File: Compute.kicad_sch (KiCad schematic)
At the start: 11 parts, among them J1 Conn_ARM_JTAG_SWD_10, U3 STM32C542CCT6, Y2 32.768kHz

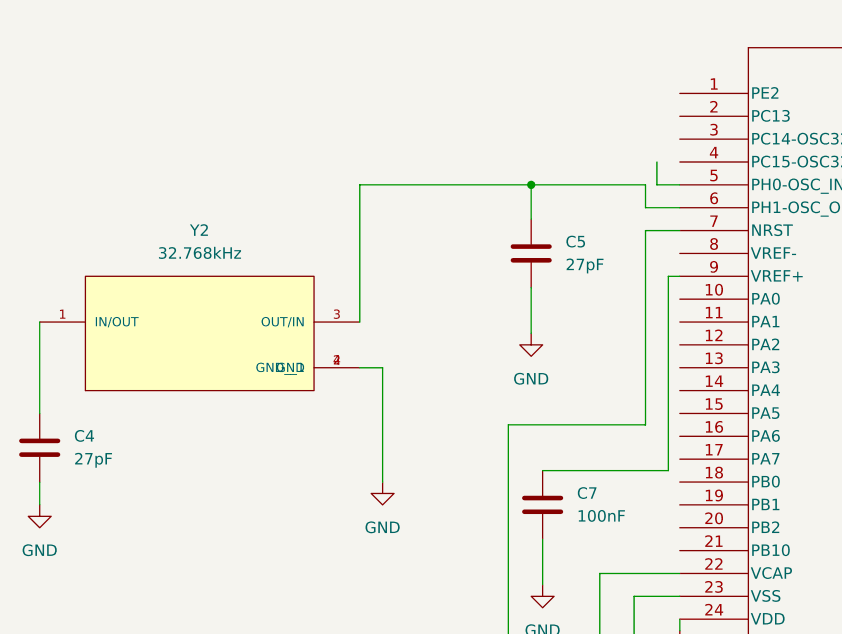
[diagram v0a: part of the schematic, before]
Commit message: fixed stuff
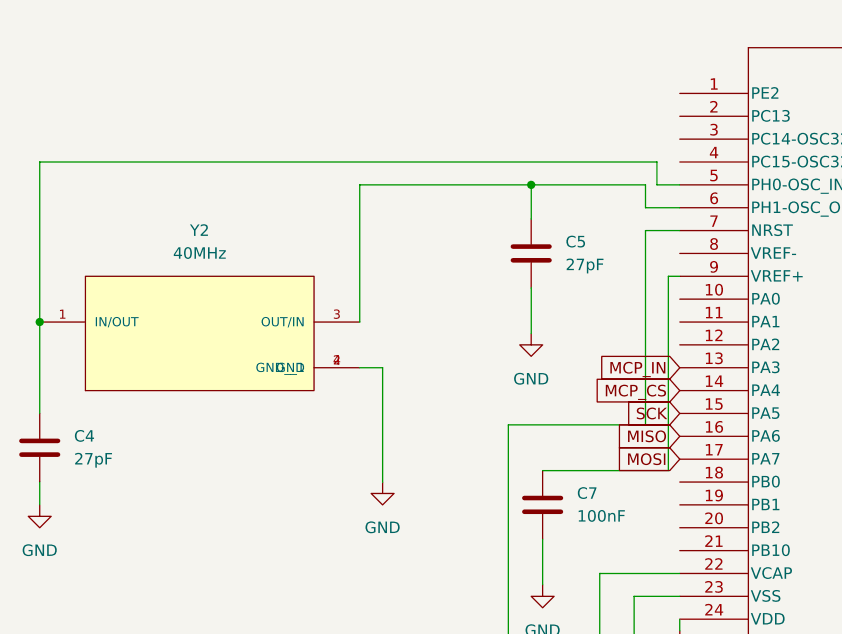
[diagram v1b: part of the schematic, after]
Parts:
- Y2: value 32.768kHz -> 40MHz
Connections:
- net MCP_IN: now reaches U3.13 (PA3)
- net MCP_CS: now reaches U3.14 (PA4)
- net SCK: now reaches U3.15 (PA5)
- net MISO: now reaches U3.16 (PA6)
- net MOSI: now reaches U3.17 (PA7)
- net at U3.5 (PH0-OSC_IN): now also C4.1, Y2.1 (IN/OUT)
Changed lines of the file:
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@@
+	)
+	(junction
+		(at 41.91 68.58)
+		(diameter 0)
+		(color 0 0 0 0)
 	)
 	(junction
@@
 	(wire
 		(pts
+			(xy 110.49 53.34) (xy 113.03 53.34)
+		)
+		(stroke
+			(width 0)
+			(type default)
+		)
+	)
+	(wire
+		(pts
 			(xy 97.79 85.09) (xy 111.76 85.09)
 		)
@@
 	(wire
 		(pts
+			(xy 110.49 50.8) (xy 110.49 53.34)
+		)
+		(stroke
+			(width 0)
+			(type default)
+		)
+	)
+	(wire
+		(pts
 			(xy 184.15 45.72) (xy 194.31 45.72)
 		)
@@
 	(wire
 		(pts
-			(xy 110.49 53.34) (xy 113.03 53.34)
-		)
-		(stroke
-			(width 0)
-			(type default)
-		)
-	)
-	(wire
-		(pts
-			(xy 110.49 50.8) (xy 110.49 53.34)
-		)
-		(stroke
-			(width 0)
-			(type default)
-		)
-	)
-	(wire
-		(pts
 			(xy 231.14 106.68) (xy 231.14 77.47)
 		)
@@
 	(wire
 		(pts
+			(xy 41.91 50.8) (xy 110.49 50.8)
+		)
+		(stroke
+			(width 0)
+			(type default)
+		)
+	)
+	(wire
+		(pts
 			(xy 184.15 76.2) (xy 186.69 76.2)
 		)
@@
 			(width 0)
 			(type default)
+		)
+	)
+	(wire
+		(pts
+			(xy 41.91 68.58) (xy 41.91 50.8)
+		)
+		(stroke
+			(width 0)
+			(type default)
+		)
+	)
+	(global_label "MCP_CS"
+		(shape input)
+		(at 113.03 76.2 180)
+		(fields_autoplaced yes)
+		(effects
+			(font
+				(size 1.27 1.27)
+			)
+			(justify right)
+		)
+		(property "Intersheetrefs" "${INTERSHEET_REFS}"
+			(at 102.6063 76.2 0)
+			(hide yes)
+			(show_name no)
+			(do_not_autoplace no)
+			(effects
+				(font
+					(size 1.27 1.27)
+				)
+				(justify right)
+			)
 		)
 	)
@@
 		)
 	)
+	(global_label "MCP_IN"
+		(shape input)
+		(at 113.03 73.66 180)
+		(fields_autoplaced yes)
+		(effects
+			(font
+				(size 1.27 1.27)
+			)
+			(justify right)
+		)
+		(property "Intersheetrefs" "${INTERSHEET_REFS}"
+			(at 103.1505 73.66 0)
+			(hide yes)
+			(show_name no)
+			(do_not_autoplace no)
+			(effects
+				(font
+					(size 1.27 1.27)
+				)
+				(justify right)
+			)
+		)
+	)
+	(global_label "MISO"
+		(shape input)
+		(at 113.03 81.28 180)
+		(fields_autoplaced yes)
+		(effects
+			(font
+				(size 1.27 1.27)
+			)
+			(justify right)
+		)
+		(property "Intersheetrefs" "${INTERSHEET_REFS}"
+			(at 105.4486 81.28 0)
+			(hide yes)
+			(show_name no)
+			(do_not_autoplace no)
+			(effects
+				(font
+					(size 1.27 1.27)
+				)
+				(justify right)
+			)
+		)
+	)
 	(global_label "CAN_RX"
 		(shape input)
@@
 				)
 				(justify left)
+			)
+		)
+	)
+	(global_label "MOSI"
+		(shape input)
+		(at 113.03 83.82 180)
+		(fields_autoplaced yes)
+		(effects
+			(font
+				(size 1.27 1.27)
+			)
+			(justify right)
+		)
+		(property "Intersheetrefs" "${INTERSHEET_REFS}"
+			(at 105.4486 83.82 0)
+			(hide yes)
+			(show_name no)
+			(do_not_autoplace no)
+			(effects
+				(font
+					(size 1.27 1.27)
+				)
+				(justify right)
+			)
+		)
+	)
+	(global_label "SCK"
+		(shape input)
+		(at 113.03 78.74 180)
+		(fields_autoplaced yes)
+		(effects
+			(font
+				(size 1.27 1.27)
+			)
+			(justify right)
+		)
+		(property "Intersheetrefs" "${INTERSHEET_REFS}"
+			(at 106.2953 78.74 0)
+			(hide yes)
+			(show_name no)
+			(do_not_autoplace no)
+			(effects
+				(font
+					(size 1.27 1.27)
+				)
+				(justify right)
 			)
 		)
@@
 			)
 		)
-		(property "Value" "32.768kHz"
+		(property "Value" "40MHz"
 			(at 59.69 60.96 0)
 			(show_name no)

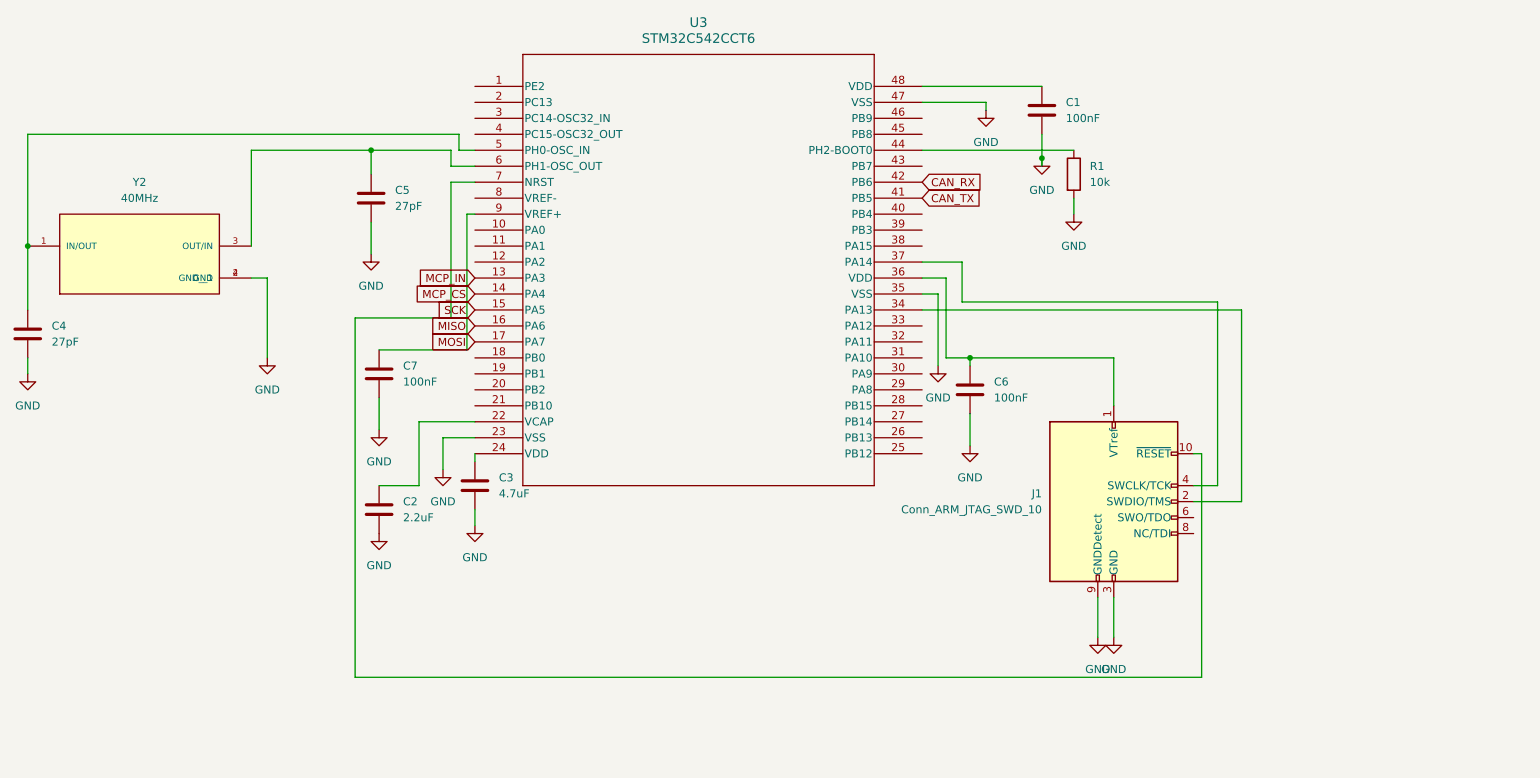
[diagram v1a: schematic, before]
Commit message: more fixes
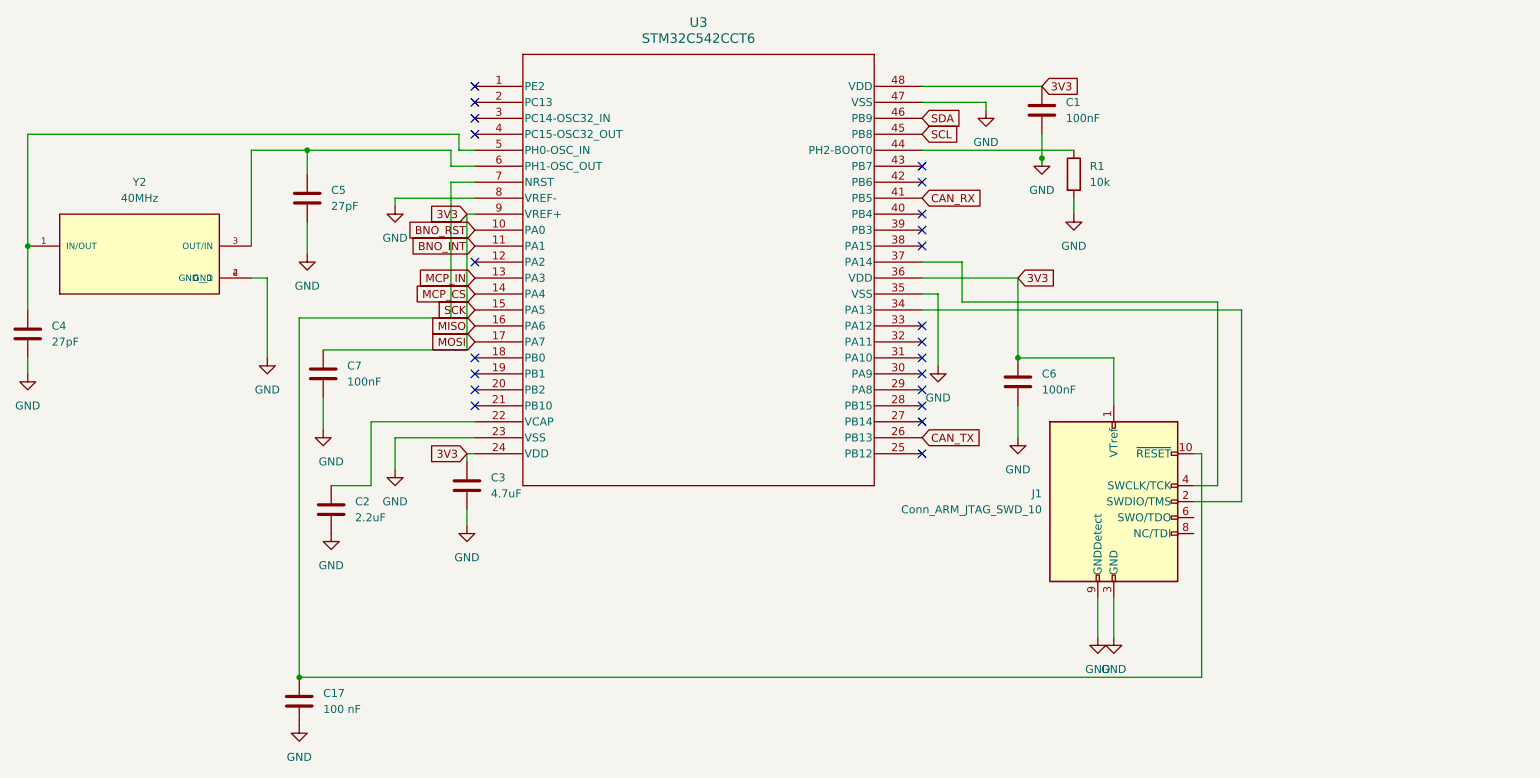
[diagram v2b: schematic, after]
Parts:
- added C17: 100 nF, symbol Device:C
- C1, C2, C3, C4, C5: footprint rov_power:SOT-23-5_MC_MCH -> Capacitor_SMD:C_0201_0603Metric
- C6, C7: footprint (none) -> Capacitor_SMD:C_0201_0603Metric
- J1: footprint (none) -> Connector_PinHeader_1.27mm:PinHeader_2x05_P1.27mm_Vertical
- R1: footprint rov_logic:LQFP48-7X7 -> Resistor_SMD:R_0201_0603Metric
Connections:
- net CAN_RX: now also U3.41 (PB5); no longer U3.42 (PB6)
- net CAN_TX: now also U3.26 (PB13); no longer U3.41 (PB5)
- net GND: now also U3.8 (VREF-), C17.2
- net 3V3: now reaches C7.1, U3.9 (VREF+)
- net 3V3: now also C1.1, C3.1, C6.1, J1.1 (VTref), U3.24 (VDD), U3.36 (VDD), U3.48 (VDD)
- net BNO_RST: now reaches U3.10 (PA0)
- net BNO_INT: now reaches U3.11 (PA1)
- net SCL: now reaches U3.45 (PB8)
- net SDA: now reaches U3.46 (PB9)
- net at J1.10 (~{RESET}), U3.7 (NRST): now also C17.1
- no-connect marks 0 -> 22
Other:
- moved on the sheet: C2, C3, C5, C6, C7

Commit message: i did stuff
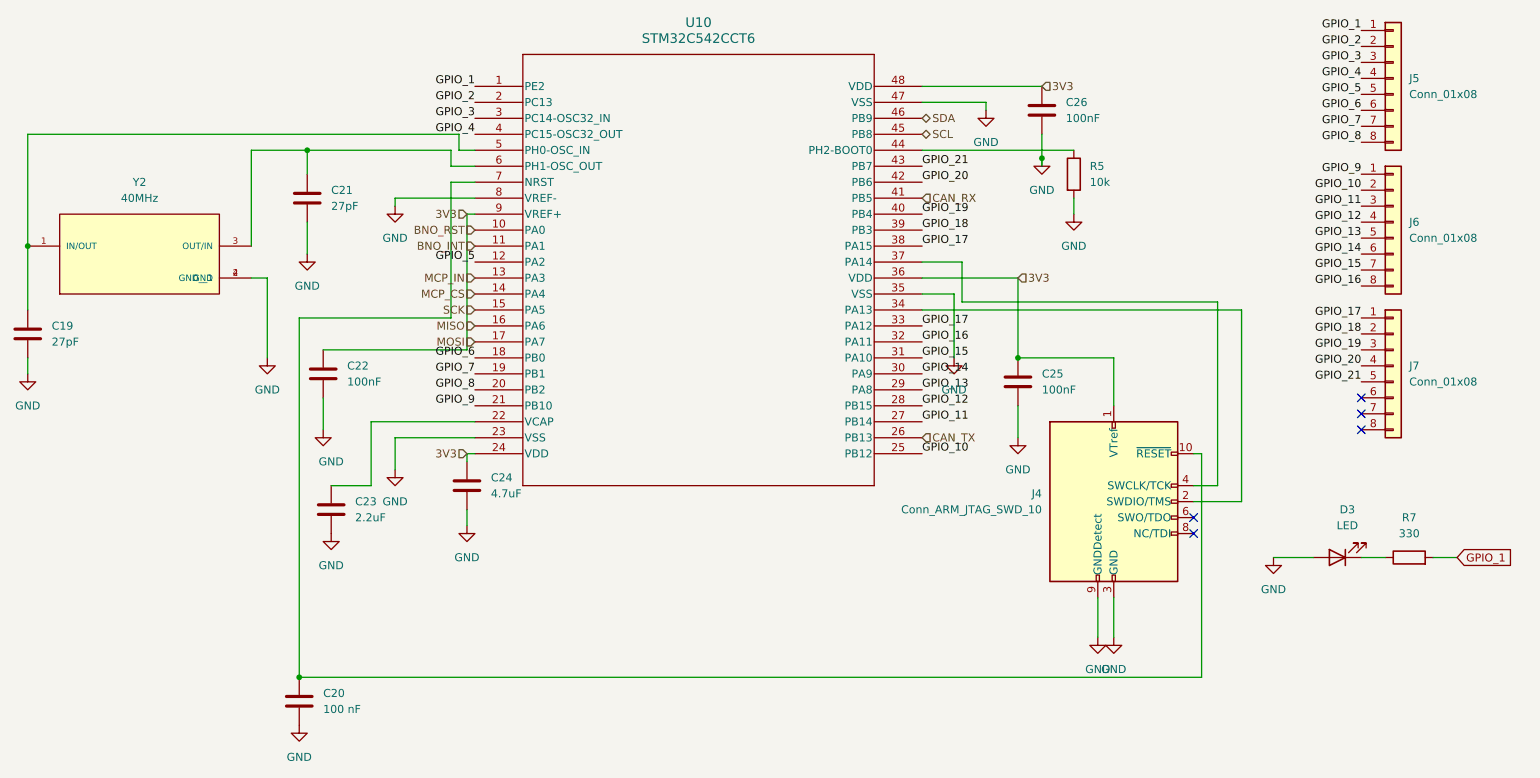
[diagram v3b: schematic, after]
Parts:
- added D3: LED, symbol Device:LED
- added J5, J6, J7: Conn_01x08, Package_DFN_QFN:DFN-8-1EP_3x2mm_P0.5mm_EP1.7x1.4mm, symbol Connector_Generic:Conn_01x08
- added R7: 330, symbol Device:R
- renumbered C4 to C19, C17 to C20, C5 to C21, C7 to C22, C2 to C23, C3 to C24, C6 to C25, C1 to C26, J1 to J4, R1 to R5, U3 to U10
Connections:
- net GND: now also D3.2 (A)
- net GPIO_1: now reaches U10.1 (PE2)
- net GPIO_1: now also J5.1 (Pin_1), R7.2
- net GPIO_5: now reaches U10.12 (PA2)
- net GPIO_5: now also J5.5 (Pin_5)
- net GPIO_6: now reaches U10.18 (PB0)
- net GPIO_6: now also J5.6 (Pin_6)
- net GPIO_7: now reaches U10.19 (PB1)
- net GPIO_7: now also J5.7 (Pin_7)
- net GPIO_2: now reaches U10.2 (PC13)
- net GPIO_2: now also J5.2 (Pin_2)
- net GPIO_8: now reaches U10.20 (PB2)
- net GPIO_8: now also J5.8 (Pin_8)
- net GPIO_9: now reaches U10.21 (PB10)
- net GPIO_9: now also J6.1 (Pin_1)
- net GPIO_10: now reaches U10.25 (PB12)
- net GPIO_10: now also J6.2 (Pin_2)
- net GPIO_11: now reaches U10.27 (PB14)
- net GPIO_11: now also J6.3 (Pin_3)
- net GPIO_12: now reaches U10.28 (PB15)
- net GPIO_12: now also J6.4 (Pin_4)
- net GPIO_13: now reaches U10.29 (PA8)
- net GPIO_13: now also J6.5 (Pin_5)
- net GPIO_3: now reaches U10.3 (PC14-OSC32_IN)
- net GPIO_3: now also J5.3 (Pin_3)
- net GPIO_14: now reaches U10.30 (PA9)
- net GPIO_14: now also J6.6 (Pin_6)
- net GPIO_15: now reaches U10.31 (PA10)
- net GPIO_15: now also J6.7 (Pin_7)
- net GPIO_16: now reaches U10.32 (PA11)
- net GPIO_16: now also J6.8 (Pin_8)
- net GPIO_17: now reaches U10.33 (PA12)
- net GPIO_17: now also U10.38 (PA15), J7.1 (Pin_1)
- net GPIO_18: now reaches U10.39 (PB3)
- net GPIO_18: now also J7.2 (Pin_2)
- net GPIO_4: now reaches U10.4 (PC15-OSC32_OUT)
- net GPIO_4: now also J5.4 (Pin_4)
- net GPIO_19: now reaches U10.40 (PB4)
- net GPIO_19: now also J7.3 (Pin_3)
- net GPIO_20: now reaches U10.42 (PB6)
- net GPIO_20: now also J7.4 (Pin_4)
- net GPIO_21: now reaches U10.43 (PB7)
- net GPIO_21: now also J7.5 (Pin_5)
- new net: D3.1 (K), R7.1
- no-connect marks 22 -> 5
